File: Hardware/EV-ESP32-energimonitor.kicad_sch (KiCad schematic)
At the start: 6 parts, among them J1 Conn_01x04_Socket

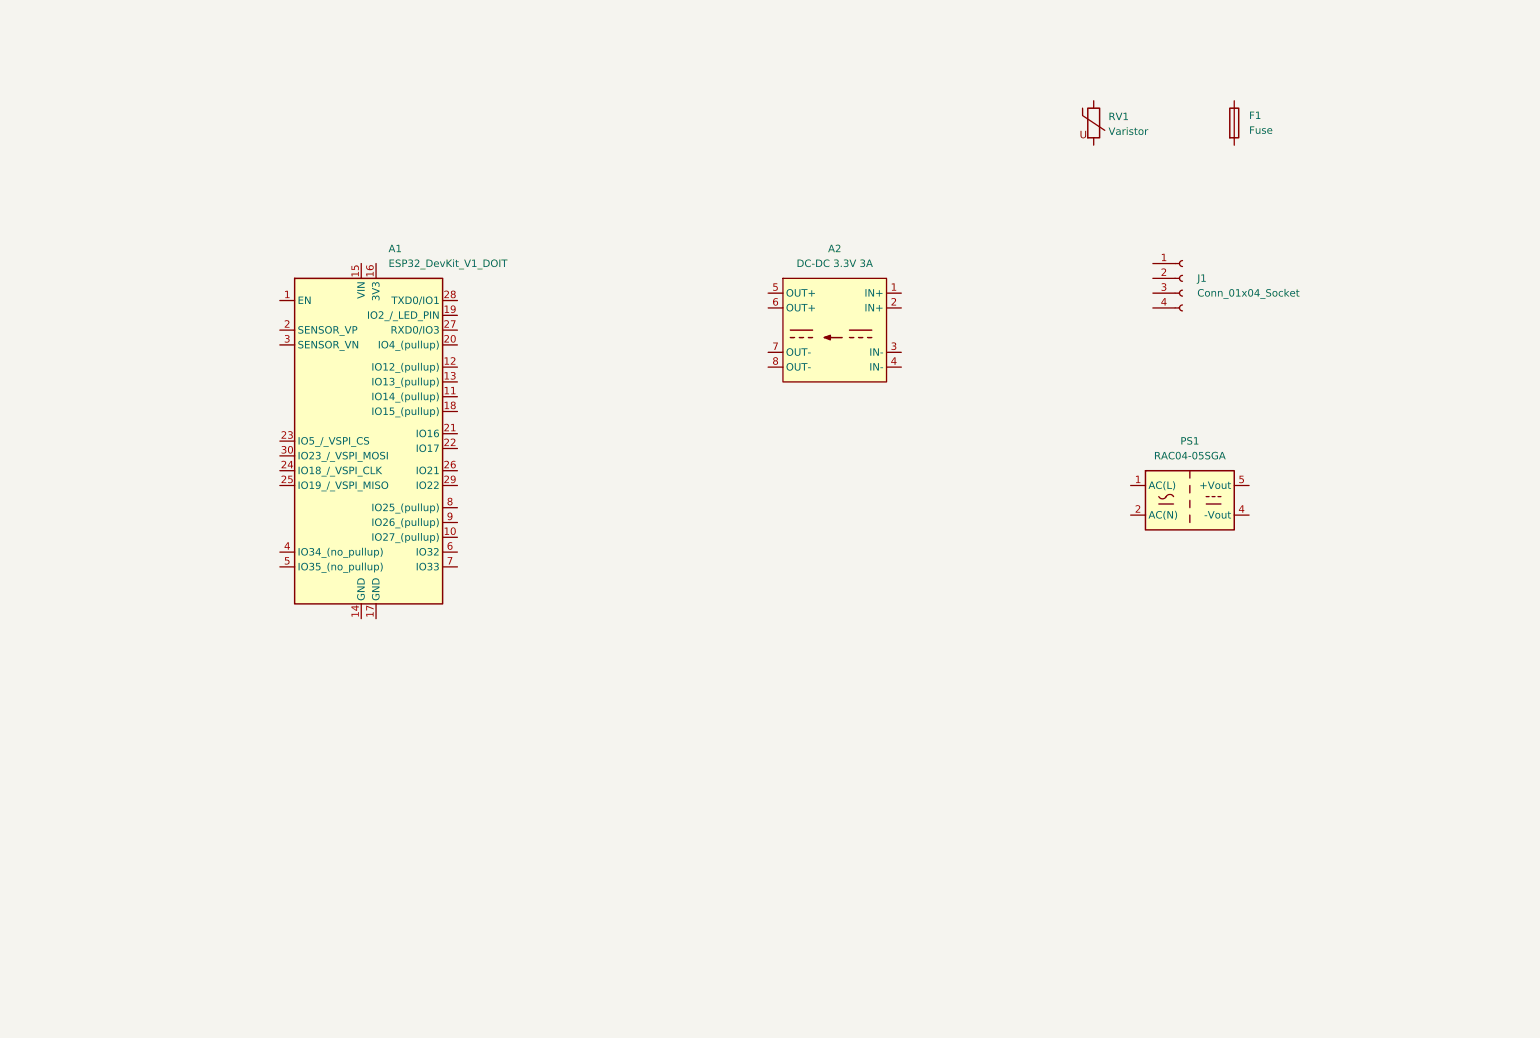
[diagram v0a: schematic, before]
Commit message: HW: diagram added
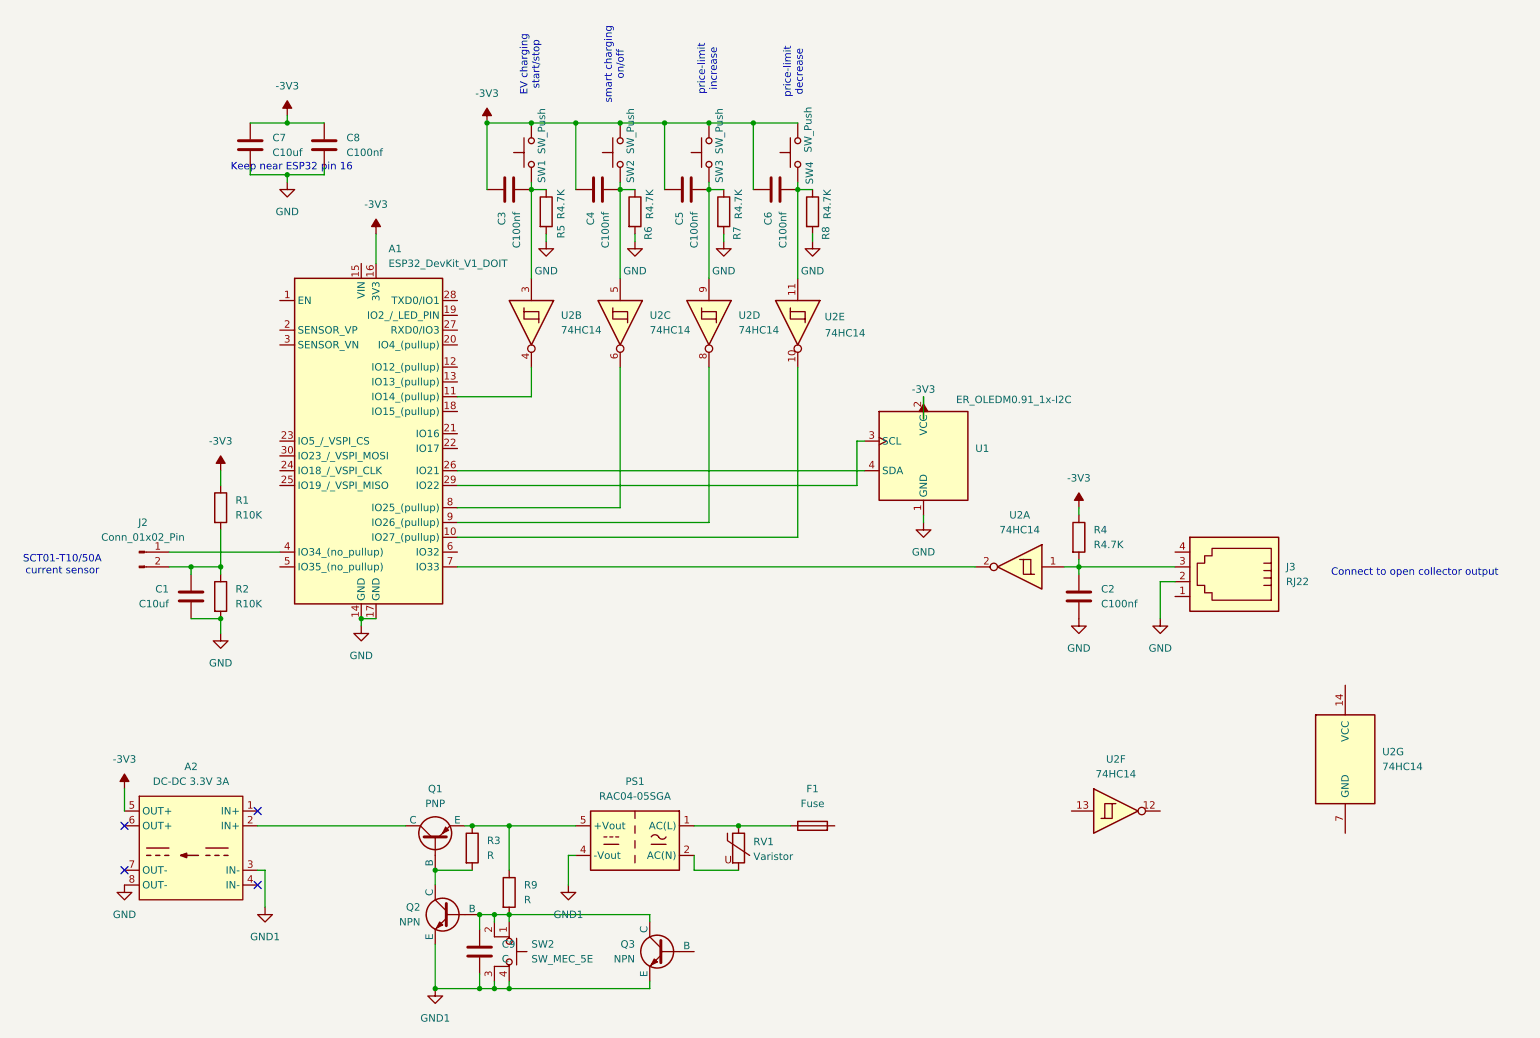
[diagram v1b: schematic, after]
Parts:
- removed J1: Conn_01x04_Socket, symbol Connector:Conn_01x04_Socket
- added C1, C7: C10uf, Capacitor_SMD:C_0603_1608Metric, symbol Local_Device_Library:C10uf
- added C2, C3, C4, C5, C6, C8: C100nf, Capacitor_SMD:C_0402_1005Metric, symbol Local_Device_Library:C100nf
- added C9: C, symbol Device:C
- added J2: Conn_01x02_Pin, symbol Connector:Conn_01x02_Pin
- added J3: RJ22, symbol Connector:RJ22
- added Q1: PNP, symbol Simulation_SPICE:PNP
- added Q2, Q3: NPN, symbol Simulation_SPICE:NPN
- added R1, R2: R10K, Resistor_SMD:R_0402_1005Metric, symbol Local_Device_Library:R10K
- added R3, R9: R, symbol Device:R
- added R4, R5, R6, R7, R8: R4.7K, Resistor_SMD:R_0402_1005Metric, symbol Local_Device_Library:R4.7K
- added SW1, SW2, SW3, SW4: SW_Push, symbol Switch:SW_Push
- added SW2: SW_MEC_5E, symbol Switch:SW_MEC_5E
- added U1: ER_OLEDM0.91_1x-I2C, Display:ER_OLEDM0.91_1x-I2C, symbol Display_Graphic:ER_OLEDM0.91_1x-I2C
- added U2: 74HC14, Package_SO:SOIC-14_3.9x8.7mm_P1.27mm, symbol Local_Miscellaneous_Library:74HC14-local_74HCxx
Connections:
- net at PS1.1 (AC(L)): now also F1.1, RV1.1
- net at PS1.2 (AC(N)): now also RV1.2
- net GND1: now reaches PS1.4 (-Vout)
- net GND1: now also A2.3 (IN-), C9.2, Q2.3 (E), Q3.3 (E), SW2.3 (K), SW2.4 (A)
- net at PS1.5 (+Vout): now also Q1.3 (E), R3.1, R9.1
- net at A2.2 (IN+): now also Q1.1 (C)
- net -3V3: now reaches A2.5 (OUT+)
- net -3V3: now also A1.16 (3V3), C3.1, C4.1, C5.1, C6.1, C7.1, C8.1, R1.1, R4.1, SW1.2, SW2.2, SW3.2, SW4.2, U1.2 (VCC)
- net GND: now reaches A2.8 (OUT-)
- net GND: now also A1.14 (GND), A1.17 (GND), C1.2, C2.2, C7.2, C8.2, J3.2, R2.2, R5.2, R6.2, R7.2, R8.2, U1.1 (GND)
- net at A1.10 (IO27_(pullup)): now also U2.10
- net at A1.11 (IO14_(pullup)): now also U2.4
- net at A1.26 (IO21): now also U1.4 (SDA)
- net at A1.29 (IO22): now also U1.3 (SCL)
- net at A1.4 (IO34_(no_pullup)): now also J2.1 (Pin_1)
- net at A1.7 (IO33): now also U2.2
- net at A1.8 (IO25_(pullup)): now also U2.6
- net at A1.9 (IO26_(pullup)): now also U2.8
- new net: Q1.2 (B), Q2.1 (C), R3.2
- new net: C5.2, R7.1, SW3.1, U2.9
- new net: C9.1, Q2.2 (B), Q3.1 (C), R9.2, SW2.1, SW2.2
- new net: C4.2, R6.1, SW2.1, U2.5
- new net: C1.1, J2.2 (Pin_2), R1.2, R2.1
- new net: C3.2, R5.1, SW1.1, U2.3
- new net: C2.1, J3.3, R4.2, U2.1
- new net: C6.2, R8.1, SW4.1, U2.11
- no-connect marks 0 -> 4
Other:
- note added: "Connect to open collector output"
- note added: "EV charging start/stop"
- note added: "Keep near ESP32 pin 16"
- note added: "SCT01-T10/50A current sensor"
- note added: "price-limit decrease"
- note added: "price-limit increase"
- note added: "smart charging on/off"
- moved on the sheet: A2, F1, PS1, RV1
